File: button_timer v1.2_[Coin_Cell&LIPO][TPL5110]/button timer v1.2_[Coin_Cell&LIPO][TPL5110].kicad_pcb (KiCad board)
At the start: 2 copper layers, 21 x 51.6 mm, 27 parts, among them J1 Conn_01x05_Female, Q1 TSM2301ACX, SW1 SW_Push, SW2 SW_Push, U1 TPS61097A, U2 AP2112K-3.3, U3 TPL5110, X1 ESP-12E

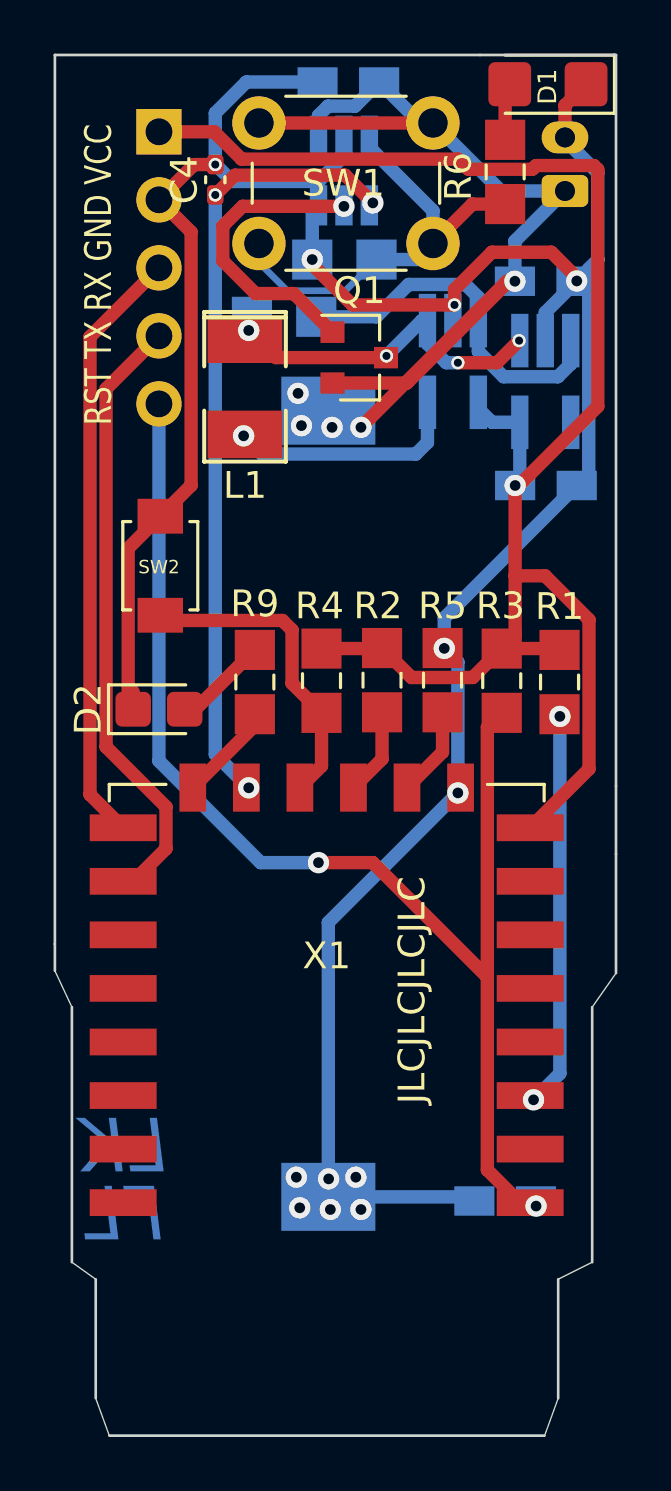
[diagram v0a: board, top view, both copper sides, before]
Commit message: Silkscreen Update
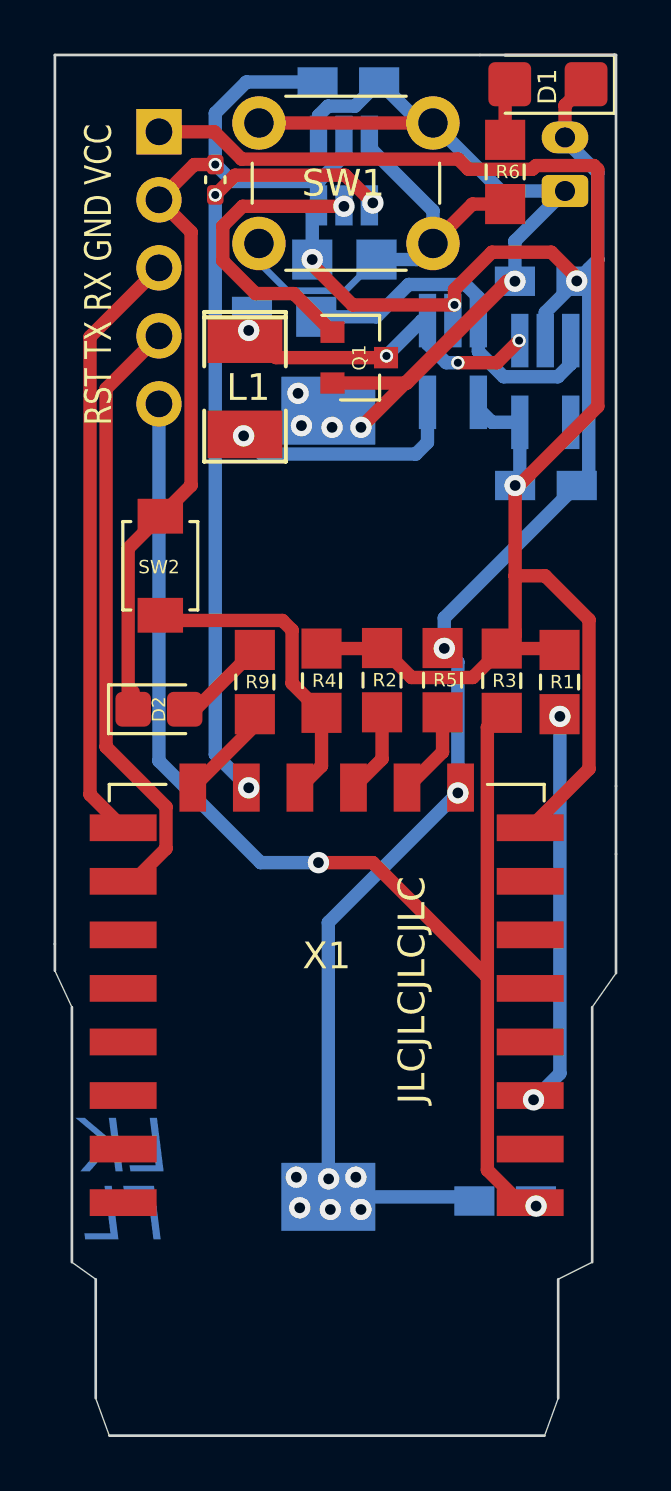
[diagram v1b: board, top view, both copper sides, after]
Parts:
- D2: footprint LED_SMD:LED_0805_2012Metric_Castellated -> handsolder:LED_0805_2012Metric_Castellated_mod
- Q1: footprint Package_TO_SOT_SMD:SOT-23 -> handsolder:SOT-23_mod
